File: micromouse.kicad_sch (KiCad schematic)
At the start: 0 parts

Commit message: schematic
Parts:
- added BT1: 7.4v, symbol Device:Battery_Cell
- added SW1: SW_SPDT_312, symbol Switch:SW_SPDT_312
- added SW2: SW_Push, symbol Switch:SW_Push
- added U1: ~, symbol stm 32 black pill:STM32F411CEU6_
- added U2: ROB-14450, ROB-14450:MODULE_ROB-14450, symbol tb6612fng:ROB-14450
- added U3, U4, U5: VL53L0X, VL53L0X:SENSOR_VL53L0X, symbol time of flight VL53L0X:VL53L0X
- added U6: ~, symbol mpu 6050:mpu_6050
- added U7, U8: ~, symbol encoder motor:encoder_motor
- added U9: ~, symbol buck:buck
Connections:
- new net 3.3v: U1. (VB), U3. (~{XSHUT}), U4. (~{XSHUT}), U5. (~{XSHUT}), U6. (vcc), U7. (motor_vcc), U8. (motor_vcc)
- new net 5v: U1. (VB), U2.2 (VCC), U9. (OUT-)
- new net 7.4v: SW1.3 (A), U2.1 (VM), U9. (OUT-)
- new net 7.4vb: BT1.1 (+), SW1.1 (B)
- new net AIN1: U1. (VB), U2.14 (AI1)
- new net AIN2: U1. (VB), U2.15 (AI2)
- new net BIN1: U1. (VB), U2.12 (BI1)
- new net BIN2: U1. (VB), U2.11 (BI2)
- new net GND: BT1.2 (-), SW1.2 (C), SW2.2, U1. (VB), U2.3 (GND), U2.5 (A02), U2.6 (B02), U2.8 (GND), U2.9 (GND), U3. (~{XSHUT}), U4. (~{XSHUT}), U5. (~{XSHUT}), U6. (vcc), U7. (motor_vcc), U8. (motor_vcc), U9. (OUT-)
- new net PWM A: U1. (VB), U2.16 (PWMA)
- new net PWM B: U1. (VB), U2.10 (PWMB)
- new net SCL MPU: U1. (VB), U6. (vcc)
- new net SCL TOF: U1. (VB), U3. (~{XSHUT}), U4. (~{XSHUT}), U5. (~{XSHUT})
- new net SDA MPU: U1. (VB), U6. (vcc)
- new net SDA TOF: U1. (VB), U3. (~{XSHUT}), U4. (~{XSHUT}), U5. (~{XSHUT})
- new net STBY: U1. (VB), U2.13 (STBY)
- new net XSHUT 1: U1. (VB), U3. (~{XSHUT})
- new net XSHUT 2: U1. (VB), U4. (~{XSHUT})
- new net XSHUT 3: U1. (VB), U5. (~{XSHUT})
- new net encoder A1: U1. (VB), U7. (motor_vcc)
- new net encoder A2: U1. (VB), U8. (motor_vcc)
- new net encoder B1: U1. (VB), U7. (motor_vcc)
- new net encoder B2: U1. (VB), U8. (motor_vcc)
- new net motor voltage: U2.4 (A01), U2.7 (B01), U7. (motor_vcc), U8. (motor_vcc)
- new net push button: SW2.1, U1. (VB)
- no-connect marks 0 -> 25

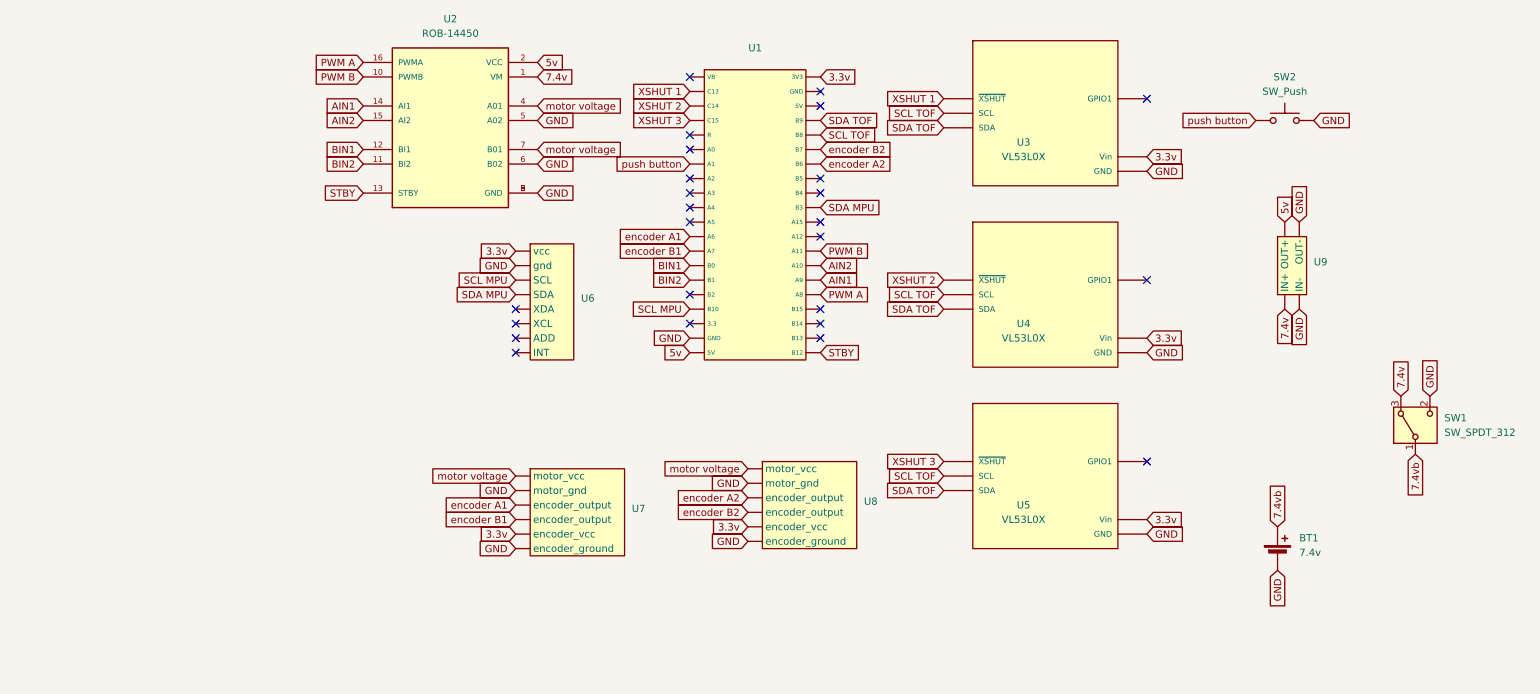
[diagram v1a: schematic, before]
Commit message: schematic changes
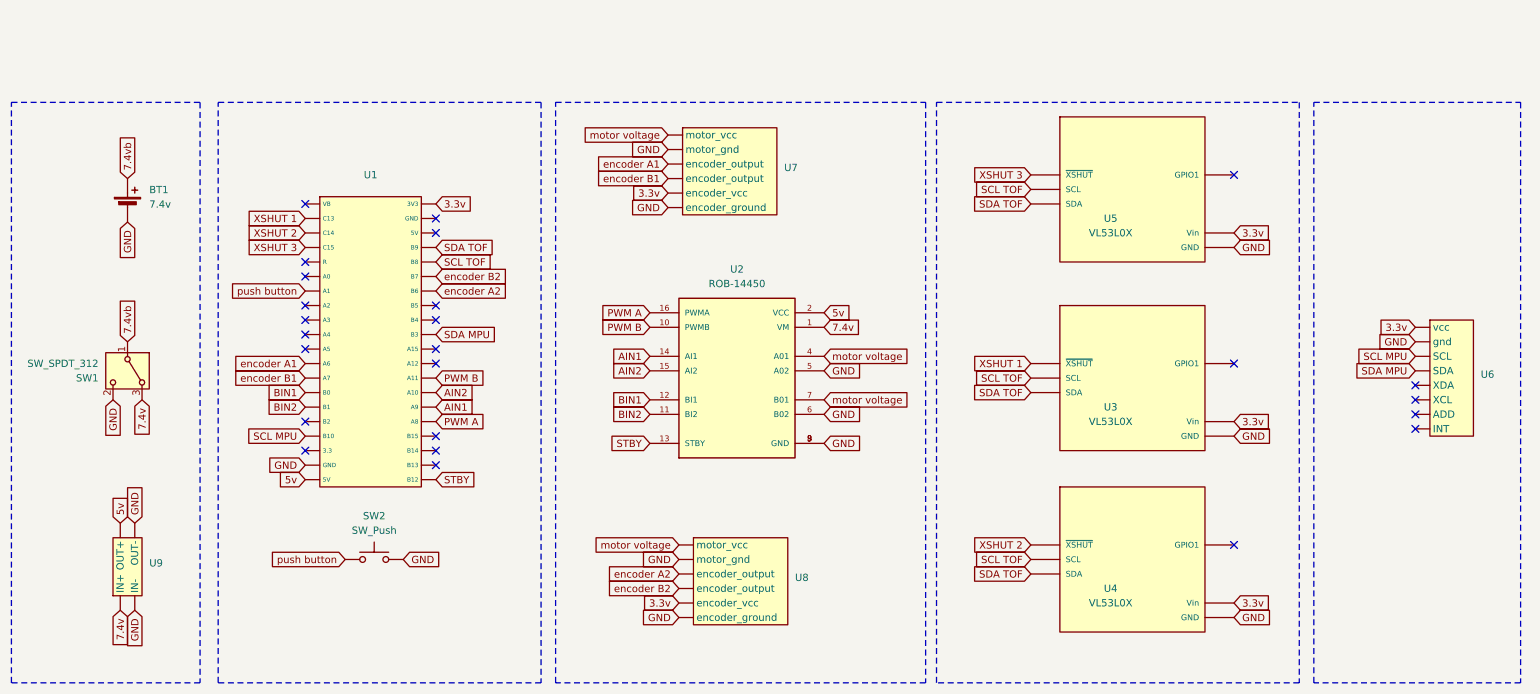
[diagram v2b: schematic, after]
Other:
- moved on the sheet: BT1, SW1, SW2, U1, U2, U3, U4, U5, U6, U7, U8, U9

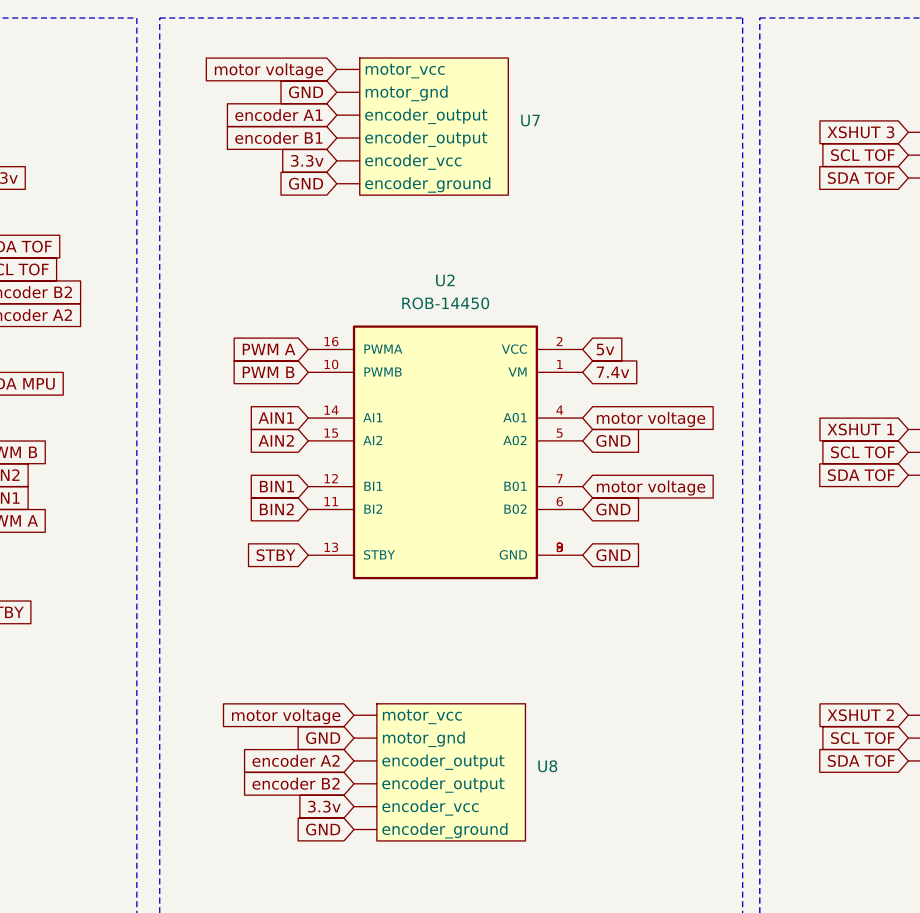
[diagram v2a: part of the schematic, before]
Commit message: schematic changes
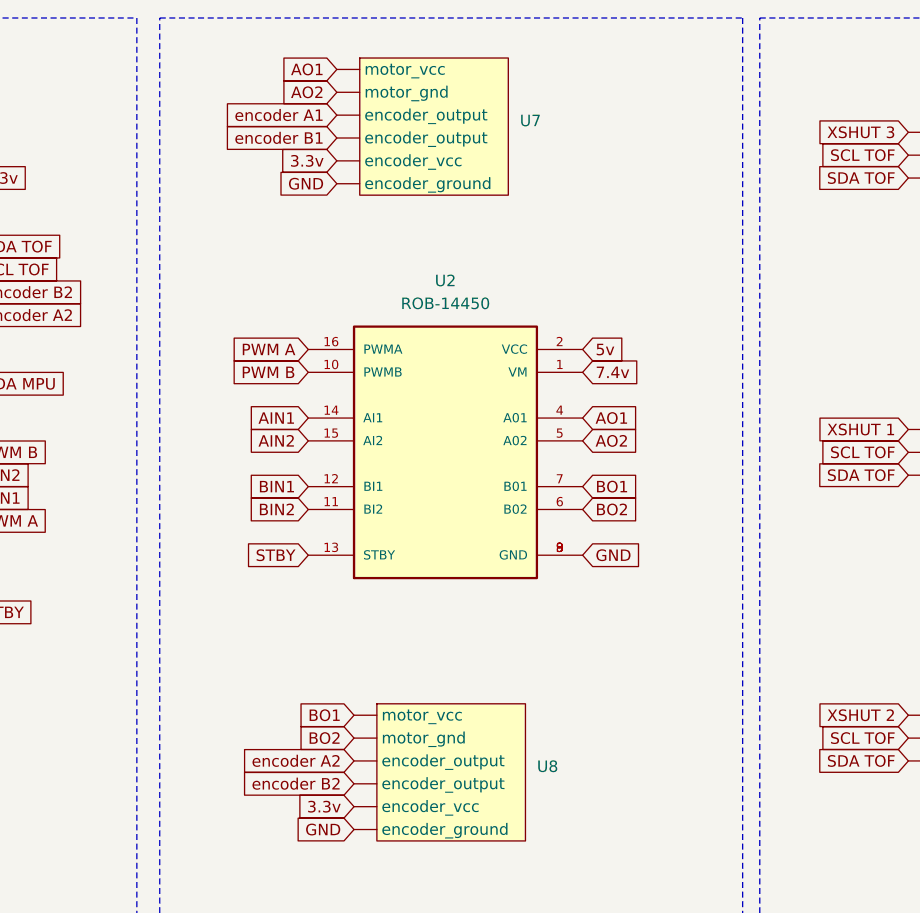
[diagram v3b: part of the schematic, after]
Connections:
- net GND: no longer U2.5 (A02), U2.6 (B02)
- removed net motor voltage: U2.4 (A01), U2.7 (B01), U7. (motor_vcc), U8. (motor_vcc)
- new net AO1: U7. (motor_vcc)
- new net AO1 : U2.4 (A01)
- new net AO2: U2.5 (A02), U7. (motor_vcc)
- new net BO1: U2.7 (B01), U8. (motor_vcc)
- new net BO2: U2.6 (B02), U8. (motor_vcc)
